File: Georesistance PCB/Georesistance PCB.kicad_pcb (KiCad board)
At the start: 4 copper layers, 70.2 x 77.5 mm, 86 parts, among them J1 Screw_Terminal_01x04, J2 Screw_Terminal_01x02, J3 Conn_01x03_Male, J4 Conn_01x11_Male, Q1 MMBF4117, Q2 MMBF4117, Q3 MMBF4117, Q4 MMBF4117, Q5 SI3430DV, Q6 SI3430DV, Q7 LNC045R090, Q8 TIP122, U1 RS8554, U10 LM350_TO220, U2 LTC6915HGN-TRPBF, U3 LM4040DBZ-2.5, U4 RS8552, U5 TXS0108EPWR, U6 ADS1115IDGS, U7 LM2776, U8 LM337L_TO92, U9 AP2127N-2.5

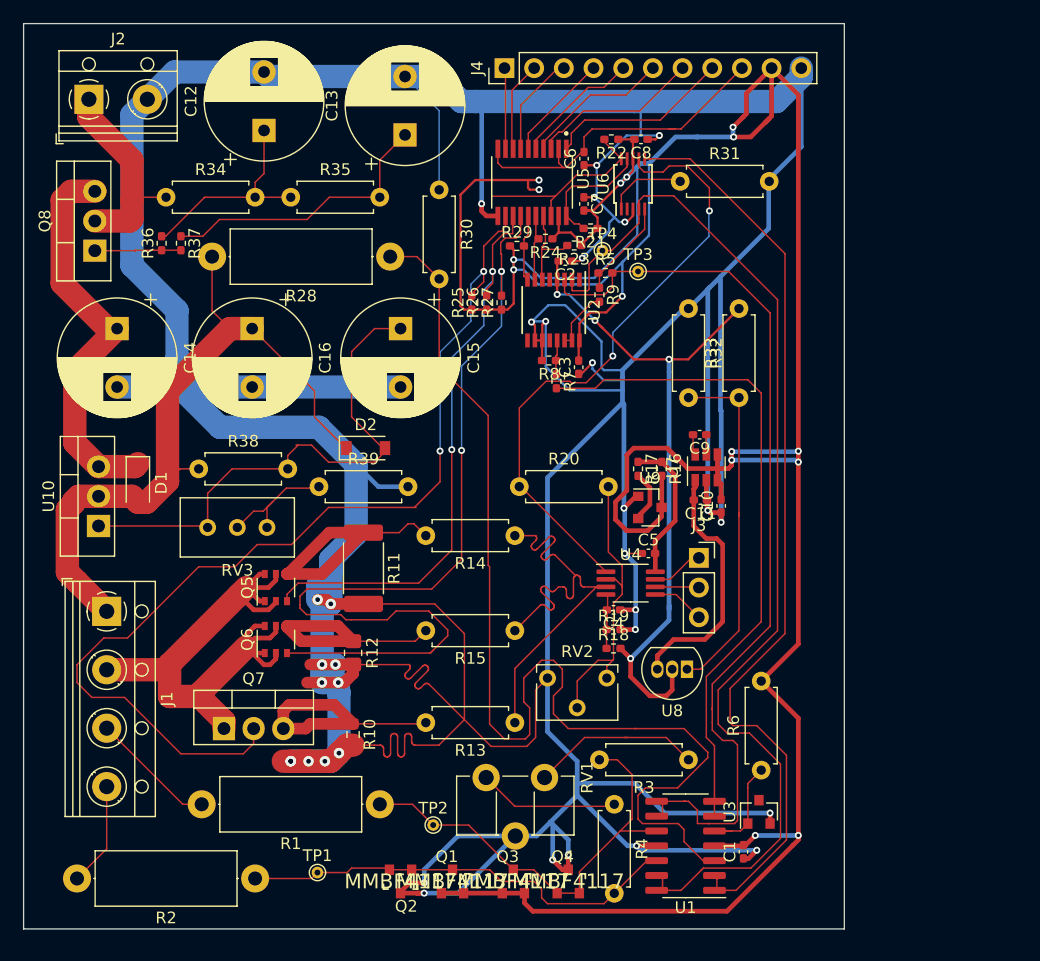
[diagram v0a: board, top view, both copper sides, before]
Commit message: added things
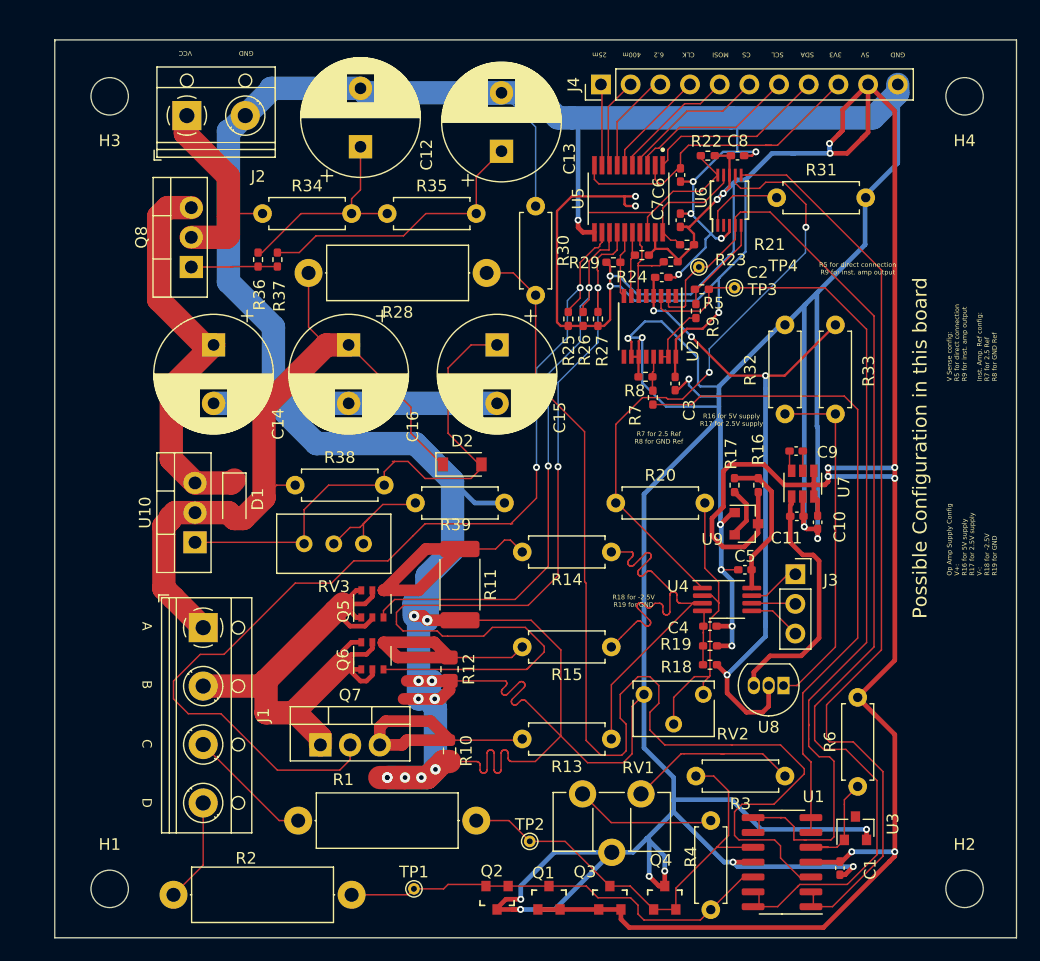
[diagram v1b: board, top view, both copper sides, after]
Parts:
- added H1: MountingHole, MountingHole:MountingHole_3.2mm_M3_DIN965, F.Cu at (20.1, 93.1)
- added H2: MountingHole, MountingHole:MountingHole_3.2mm_M3_DIN965, F.Cu at (93.2, 93.1)
- added H3: MountingHole, MountingHole:MountingHole_3.2mm_M3_DIN965, F.Cu at (20.1, 25.3)
- added H4: MountingHole, MountingHole:MountingHole_3.2mm_M3_DIN965, F.Cu at (93.2, 25.3)
- moved J2 8.50 mm to (26.7, 26.9)
- moved C11 8.37 mm to (78.9, 61.2)
- moved C8 8.37 mm to (73.8, 30.4)
- moved C9 8.37 mm to (78.8, 55.6)
- moved U6 8.37 mm to (73.1, 34.2)
- moved U9 8.37 mm to (74.5, 61.8)
- moved U8 8.37 mm to (77.7, 75.7)
- moved C12 8.37 mm to (41.5, 29.6)
- moved C13 8.37 mm to (53.6, 30.0)
- moved C15 8.37 mm to (53.2, 46.5)
- moved C2 8.37 mm to (67.3, 40.8)
- moved C3 8.37 mm to (68.5, 49.9)
- moved C6 8.37 mm to (68.9, 32.0)
- moved D1 8.37 mm to (30.7, 59.8)
- moved J4 8.37 mm to (62.1, 24.3)
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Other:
- board size 70.2 x 77.5 mm -> 82.3 x 76.8 mm
- board text added: "25m"
- board text added: "3V3"
- board text added: "400m"
- board text added: "5V"
- board text added: "6.2"
- board text added: "A"
- board text added: "B"
- board text added: "C"
- board text added: "CLK"
- board text added: "CS"
- board text added: "D"
- board text added: "GND"
- board text added: "MOSI"
- board text added: "Op Amp Supply Config V+: R16 for 5V supply R17 for 2.5V supply V-: R18 for -2.5V R19 for GND"
- board text added: "Possible Configuration in this board"
- board text added: "R16 for 5V supply R17 for 2.5V supply"
- board text added: "R18 for -2.5V R19 for GND"
- board text added: "R5 for direct connection R9 for inst. amp output"
- board text added: "R7 for 2.5 Ref R8 for GND Ref"
- board text added: "SCL"
- board text added: "SDA"
- board text added: "V Sense config: R5 for direct connection R9 for inst. amp output Inst. Amp. Ref config: R7 for 2.5 Ref R8 for GND Ref"
- board text added: "VCC"
